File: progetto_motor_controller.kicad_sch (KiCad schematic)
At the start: 38 parts, among them J1 USB_B_Micro, J2 Conn_01x06, J3 Conn_01x04, J4 Screw_Terminal_01x03, J5 Conn_01x05, J6 Conn_02x10_Counter_Clockwise, J7 Conn_01x02, Q1 BSC022N04LSATMA1, SW1 SW_SPDT, U1 STM32F303RETx, U3 USBLC6-2P6, Y1 16MHz

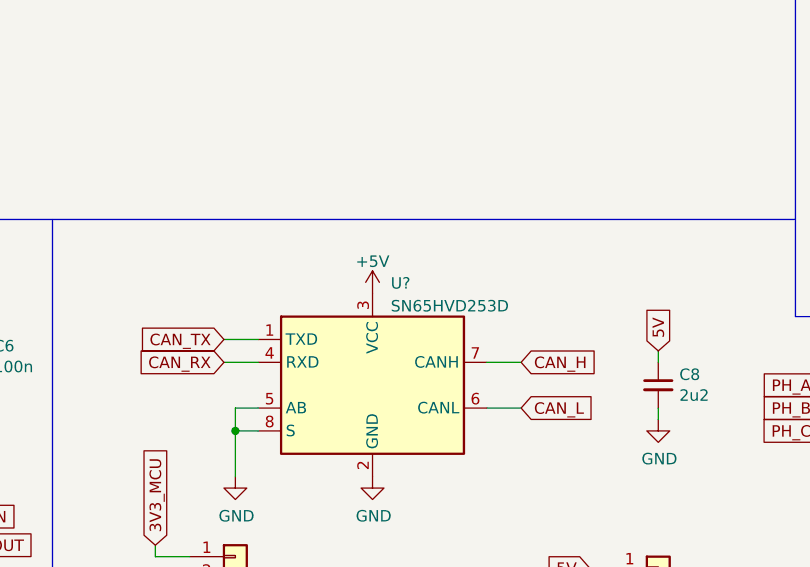
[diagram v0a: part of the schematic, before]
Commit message: Third commit
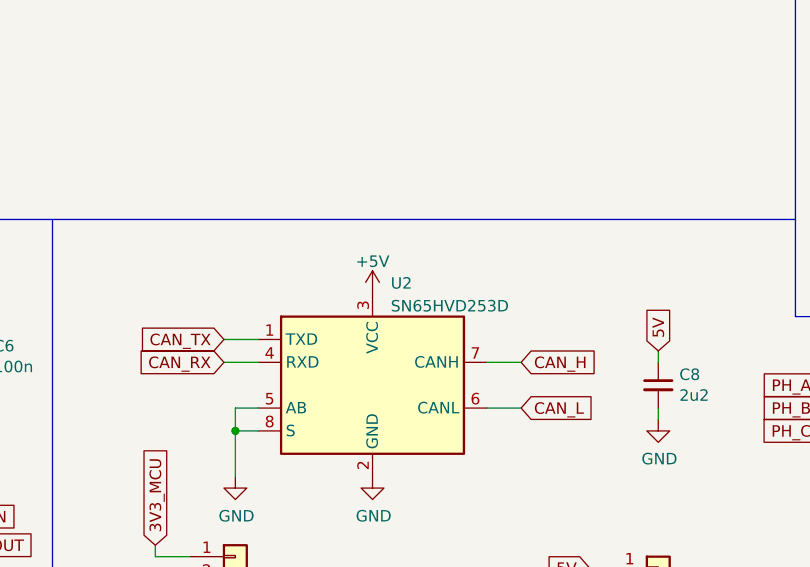
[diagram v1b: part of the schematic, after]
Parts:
- gave numbers to parts that had none: 1
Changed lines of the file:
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@@
   (symbol (lib_id "MyLibrary_PMSM:SN65HVD253D") (at 149.86 90.17 0) (unit 1)
     (in_bom yes) (on_board yes) (fields_autoplaced)
-    (property "Reference" "U?" (id 0) (at 151.8794 78.8502 0)
+    (property "Reference" "U2" (id 0) (at 151.8794 78.8502 0)
       (effects (font (size 1.27 1.27)) (justify left))
     )
@@
       (reference "U1") (unit 1) (value "STM32F303RETx") (footprint "Package_QFP:LQFP-64_10x10mm_P0.5mm")
     )
+    (path "/80b39198-0427-4a2c-87f3-1492d50638db"
+      (reference "U2") (unit 1) (value "SN65HVD253D") (footprint "Package_SO:SOIC-8_3.9x4.9mm_P1.27mm")
+    )
     (path "/00000000-0000-0000-0000-000061e1e007"
       (reference "U3") (unit 1) (value "USBLC6-2P6") (footprint "Package_TO_SOT_SMD:SOT-666")
     )
+    (path "/00000000-0000-0000-0000-000061cd02c2/612a78e7-cc68-4577-b241-2d6ade45da87"
+      (reference "U4") (unit 1) (value "TMC6140") (footprint "MyLibrary:TMC6140-LA")
+    )
     (path "/00000000-0000-0000-0000-000061cd02c2/3359e259-3a3c-4aa4-8732-3dbaa9867503"
-      (reference "U?") (unit 1) (value "TSC2011") (footprint "")
-    )
-    (path "/00000000-0000-0000-0000-000061cd02c2/612a78e7-cc68-4577-b241-2d6ade45da87"
-      (reference "U?") (unit 1) (value "TMC6140") (footprint "")
+      (reference "U5") (unit 1) (value "TSC2011") (footprint "")
+    )
+    (path "/00000000-0000-0000-0000-000061cd02c2/7c94c38e-623f-41eb-bdd6-5171cfc8b42f"
+      (reference "U6") (unit 1) (value "TSC2011") (footprint "")
+    )
+    (path "/1dc60600-5235-4456-91bf-a196642211fa/f139b3a3-5b4a-4b3f-8883-678a3f953d6f"
+      (reference "U7") (unit 1) (value "MYRGC07506_1") (footprint "MyLibrary:Murata_picoBK")
     )
     (path "/1dc60600-5235-4456-91bf-a196642211fa/7902e9cd-4be0-4e1c-b27c-519fb539f14c"
-      (reference "U?") (unit 1) (value "TLV707") (footprint "")
-    )
-    (path "/00000000-0000-0000-0000-000061cd02c2/7c94c38e-623f-41eb-bdd6-5171cfc8b42f"
-      (reference "U?") (unit 1) (value "TSC2011") (footprint "")
-    )
-    (path "/80b39198-0427-4a2c-87f3-1492d50638db"
-      (reference "U?") (unit 1) (value "SN65HVD253D") (footprint "Package_SO:SOIC-8_3.9x4.9mm_P1.27mm")
-    )
-    (path "/1dc60600-5235-4456-91bf-a196642211fa/f139b3a3-5b4a-4b3f-8883-678a3f953d6f"
-      (reference "U?") (unit 1) (value "MYRGC07506_1") (footprint "")
+      (reference "U8") (unit 1) (value "TLV707") (footprint "MyLibrary:TLV707")
     )
     (path "/00000000-0000-0000-0000-000061caf110"
